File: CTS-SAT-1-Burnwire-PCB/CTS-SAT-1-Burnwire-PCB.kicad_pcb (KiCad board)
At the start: 2 copper layers, 50.8 x 22.9 mm, 12 parts, among them J1 Molex_PicoBlade_53398-0471_1x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, J2 Molex_PicoBlade_53047-0610_1x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

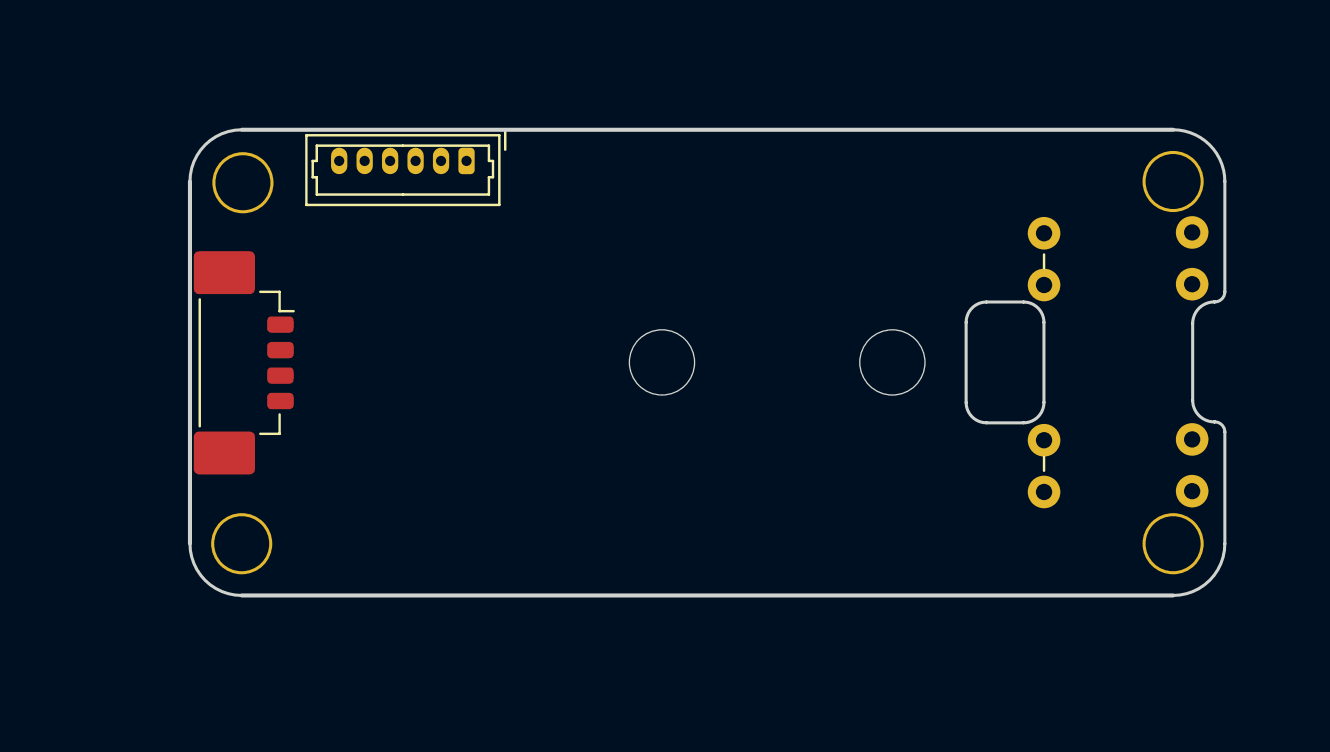
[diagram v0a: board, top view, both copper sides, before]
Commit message: Layout and routing
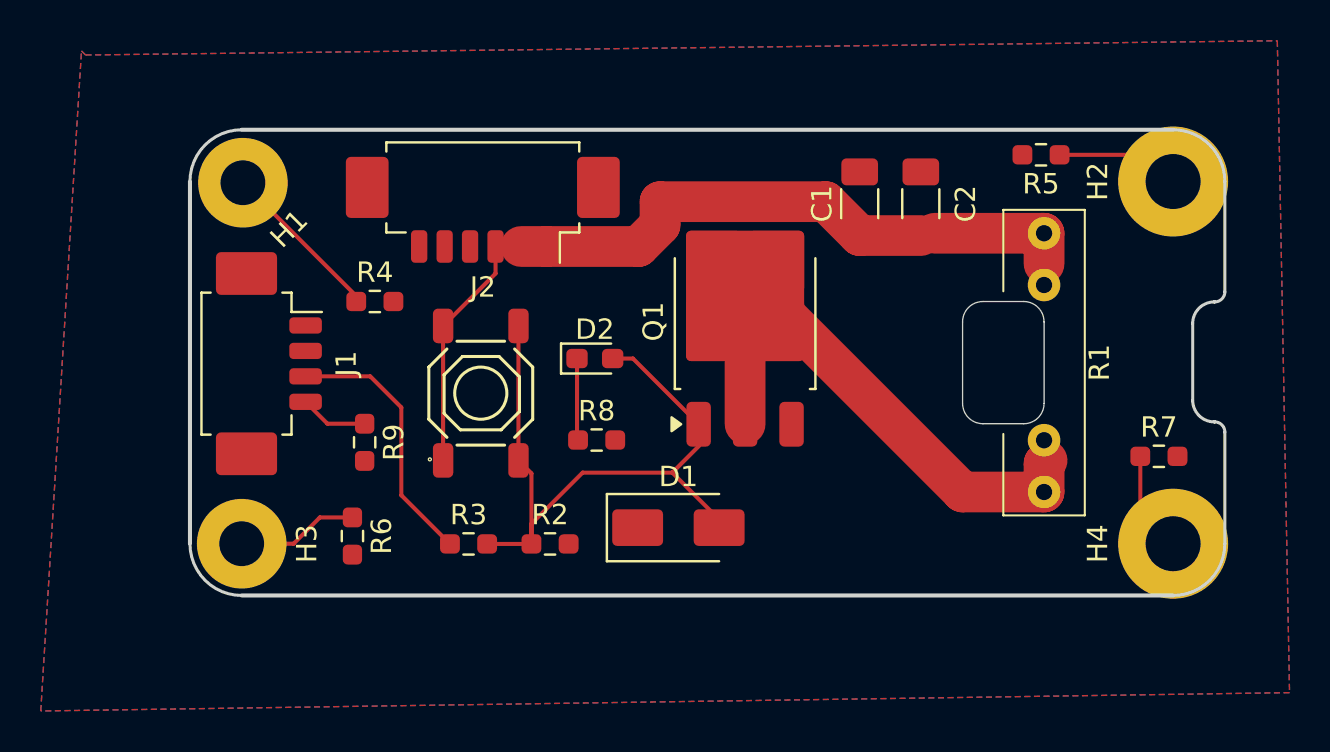
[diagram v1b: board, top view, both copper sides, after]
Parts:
- removed the R1 at (117.5, 61.5)
- removed the R1 at (117.5, 59.0)
- removed REF** (x2): MountingHole_3.2mm_M3, MountingHole:MountingHole_3.2mm_M3
- removed REF** (x3): MountingHole_2.6mm_M2.5, MountingHole:MountingHole_2.7mm_M2.5
- removed REF**: MountingHole_2.7mm_M2.5, MountingHole:MountingHole_2.7mm_M2.5
- removed REF**: R_Axial_DIN0309_L9.0mm_D3.2mm_P12.70mm_Horizontal, Resistor_THT:R_Axial_DIN0309_L9.0mm_D3.2mm_P12.70mm_Horizontal
- added C1: 10u, Capacitor_SMD:C_1206_3216Metric_Pad1.33x1.80mm_HandSolder, F.Cu at (108.5, 57.5)
- added C2: 100n, Capacitor_SMD:C_1206_3216Metric_Pad1.33x1.80mm_HandSolder, F.Cu at (111.5, 57.5)
- added D1: SMAJ13CA, Diode_SMD:D_SMA, F.Cu at (99.6, 73.4)
- added D2: LED, LED_SMD:LED_0603_1608Metric_Pad1.05x0.95mm_HandSolder, F.Cu at (95.5, 65.1)
- added H1: MountingHole_Pad, MountingHole:MountingHole_2.2mm_M2_Pad, F.Cu at (78.2, 56.5)
- added H2: MountingHole_Pad, MountingHole:MountingHole_2.7mm_M2.5_Pad, F.Cu at (123.9, 56.4)
- added H3: MountingHole_Pad, MountingHole:MountingHole_2.2mm_M2_Pad, F.Cu at (78.2, 74.2)
- added H4: MountingHole_Pad, MountingHole:MountingHole_2.7mm_M2.5_Pad, F.Cu at (123.9, 74.2)
- added Q1: IPD90N04S4L, Package_TO_SOT_SMD:TO-252-3_TabPin2, F.Cu at (102.9, 63.3)
- added R1: R, 00-footprint-lib:AxialBurnResistor, F.Cu at (117.5, 65.3)
- added R3: 100, Resistor_SMD:R_0603_1608Metric_Pad0.98x0.95mm_HandSolder, F.Cu at (89.3, 74.2)
- added R4: 0, Resistor_SMD:R_0603_1608Metric_Pad0.98x0.95mm_HandSolder, F.Cu at (84.7, 62.3)
- added R5: 0, Resistor_SMD:R_0603_1608Metric_Pad0.98x0.95mm_HandSolder, F.Cu at (117.4, 55.1)
- added R6: 0, Resistor_SMD:R_0603_1608Metric_Pad0.98x0.95mm_HandSolder, F.Cu at (83.6, 73.8)
- added R7: 0, Resistor_SMD:R_0603_1608Metric_Pad0.98x0.95mm_HandSolder, F.Cu at (123.2, 69.9)
- added R8: 5k1, Resistor_SMD:R_0603_1608Metric_Pad0.98x0.95mm_HandSolder, F.Cu at (95.6, 69.1)
- added R9: 100k, Resistor_SMD:R_0603_1608Metric_Pad0.98x0.95mm_HandSolder, F.Cu at (84.2, 69.2)
- added S1: Tactile_Button, 00-footprint-lib:SW-SMD_4P-L5.1-W5.1-P3.70-LS6.5-TL-2, F.Cu at (89.9, 66.8)
- J1: value Molex_PicoBlade_53398-0471_1x04-1MP_P1.25mm_Vertical -> Conn_01x04_MountingPin; footprint Connector_Molex:Molex_PicoBlade_53398-0471_1x04-1MP_P1.25mm_Vertical -> Connector_Molex:Molex_PicoBlade_53261-0471_1x04-1MP_P1.25mm_Horizontal
- J2: value Molex_PicoBlade_53047-0610_1x06_P1.25mm_Vertical -> Conn_01x06_MountingPin; footprint Connector_Molex:Molex_PicoBlade_53047-0610_1x06_P1.25mm_Vertical -> Connector_Molex:Molex_PicoBlade_53261-0671_1x06-1MP_P1.25mm_Horizontal
- R2: value 100 -> 5k1; footprint Resistor_THT:R_Axial_DIN0207_L6.3mm_D2.5mm_P7.62mm_Horizontal -> Resistor_SMD:R_0603_1608Metric_Pad0.98x0.95mm_HandSolder
- moved R2 34.0 mm to (93.3, 74.2), turned to 0 degrees
- moved J2 1.97 mm to (90.0, 57.2)
- moved J1 0.09 mm to (78.9, 65.3)
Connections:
- net Vin renamed VDC
- J1 pad 1: IN1 -> GND
- J1 pad 2: IN2 -> GND
- J1 pad 3: EN3V -> BURN_CTRL
- J1 pad 4: EN3V -> Net-(J1-Pin_4)
- J1 pad MP: (no net) -> GND
- R2 pad 2: +5V -> GND
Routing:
- net VDC: track 0.00 -> 40.3 mm
- net Net-(D1-A2): track 0.00 -> 34.2 mm
- net Net-(Q1-D): track 0.00 -> 26.6 mm
- net BURN_CTRL: track 0.00 -> 13.0 mm
- net Net-(H1-Pad1): track 0.00 -> 8.13 mm
- net Net-(H2-Pad1): track 0.00 -> 6.12 mm
- net Net-(H3-Pad1): track 0.00 -> 5.97 mm
- net Net-(H4-Pad1): track 0.00 -> 4.96 mm
- net Net-(D2-K): track 0.00 -> 4.02 mm
- net Net-(J1-Pin_4): track 0.00 -> 3.35 mm
- added copper zone on B.Cu, net GND
- added copper zone on F.Cu, net GND
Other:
- outline, holes or cut-outs redrawn
